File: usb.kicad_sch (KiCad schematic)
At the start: 7 parts, among them J5 USB, U6 USBLC6-2SC6

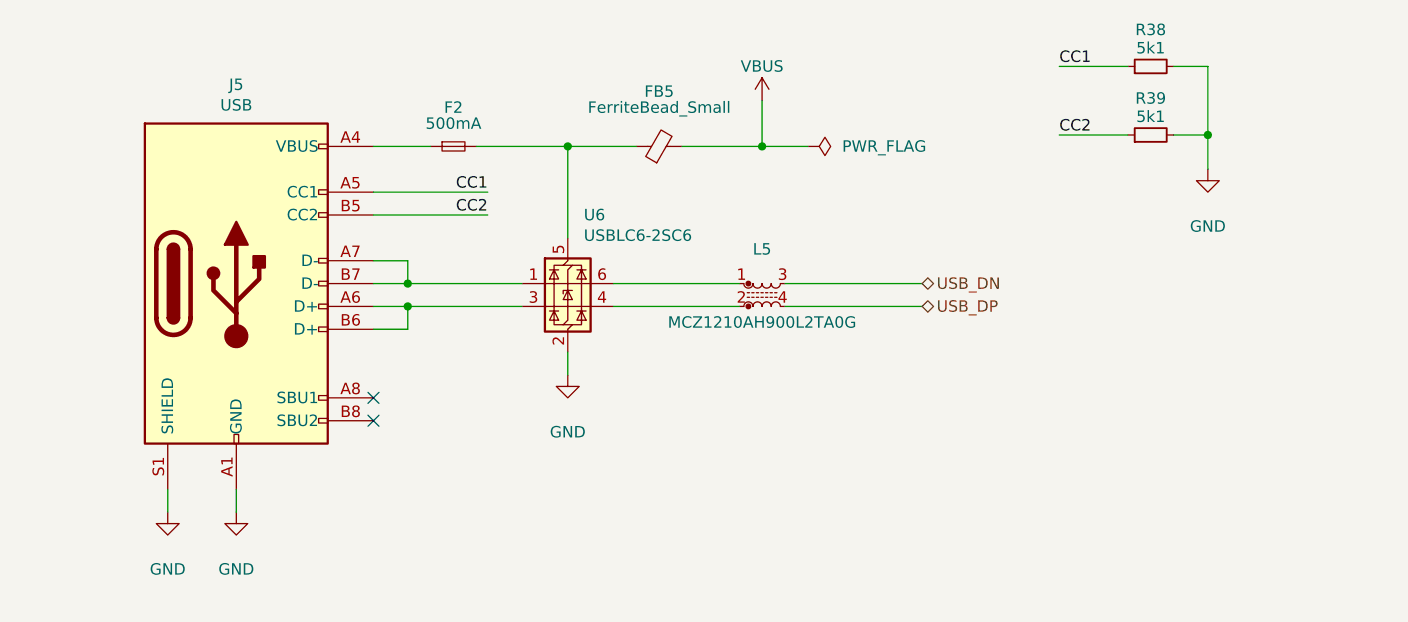
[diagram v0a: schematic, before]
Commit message: brd: routing in progress
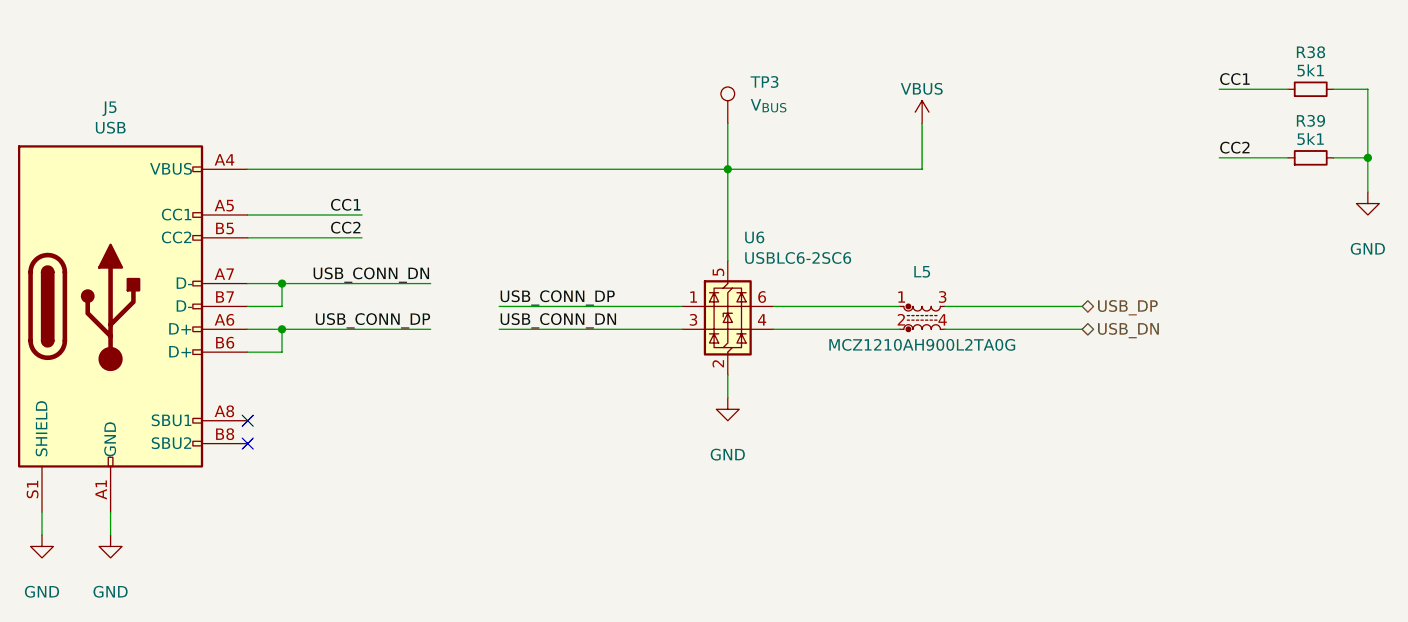
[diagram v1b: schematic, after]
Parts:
- removed F2: 500mA, Fuse:Fuse_1206_3216Metric, symbol Device:Fuse_Small
- removed FB5: FerriteBead_Small, Inductor_SMD:L_0805_2012Metric_Pad1.05x1.20mm_HandSolder, symbol Device:FerriteBead_Small
- added TP3: V_{BUS}, TestPoint:TestPoint_Pad_D1.0mm, symbol Connector:TestPoint
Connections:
- net USB_DN: now also L5.4; no longer L5.3
- net USB_DP: now also L5.3; no longer L5.4
- net VBUS: now also J5.A4 (VBUS), J5.A9 (VBUS), J5.B4 (VBUS), J5.B9 (VBUS), U6.5 (VBUS), TP3.1
- net USB_CONN_DN: now reaches J5.A7 (D-), J5.B7 (D-)
- net USB_CONN_DN: now also U6.3 (I/O2); no longer U6.1 (I/O1)
- net USB_CONN_DP: now reaches J5.A6 (D+), J5.B6 (D+)
- net USB_CONN_DP: now also U6.1 (I/O1); no longer U6.3 (I/O2)
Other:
- moved on the sheet: J5, L5, R38, R39, U6
